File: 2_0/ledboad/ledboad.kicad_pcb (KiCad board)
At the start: 2 copper layers, 96 x 34.2 mm, 334 parts, among them J1 Conn_02x05_Odd_Even, Q1 AO3401A, Q2 AO3401A, Q3 AO3401A, Q4 AO3401A, Q5 AO3401A, Q6 AO3401A, Q7 AO3401A, Q8 AO3401A, SW1 RST, U1 STM32G070CBTx, U2 XC6206PxxxMR, Y1 2016/DNP

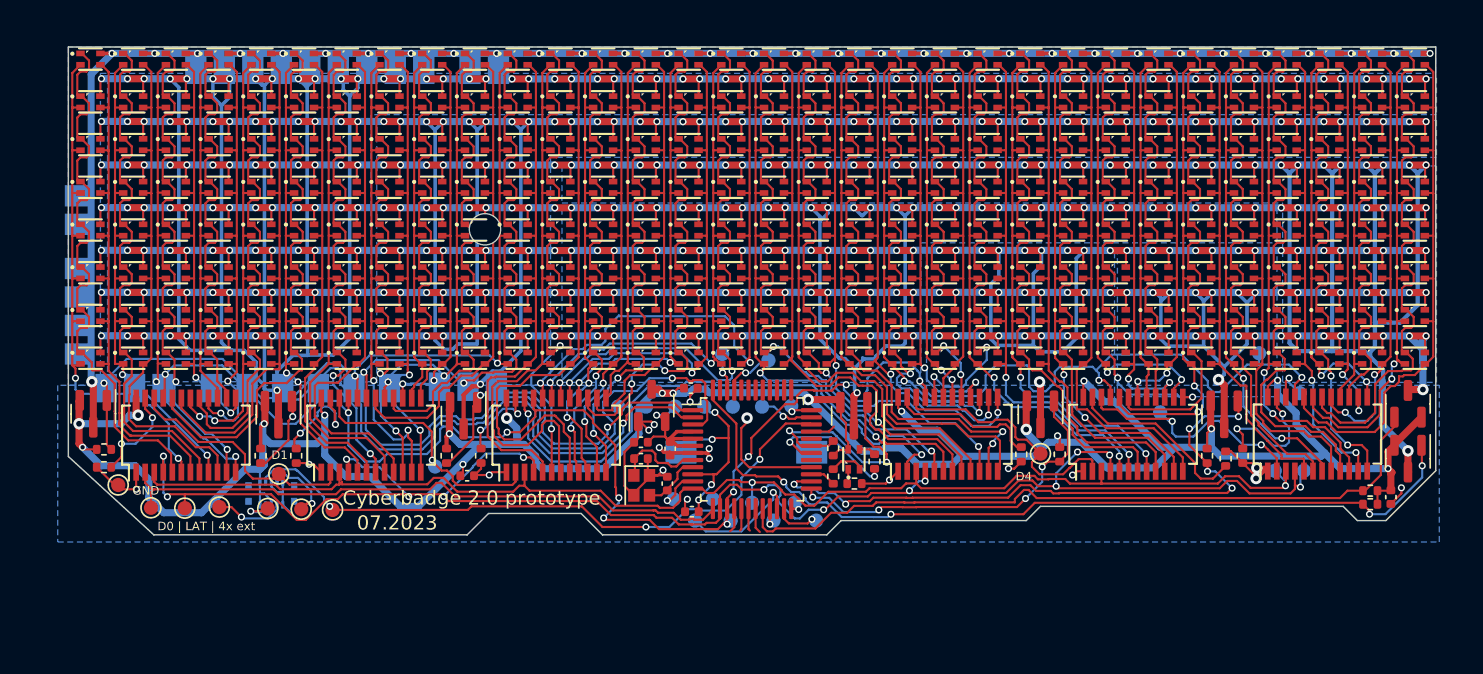
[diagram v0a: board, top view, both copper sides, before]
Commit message: commit before rescheme
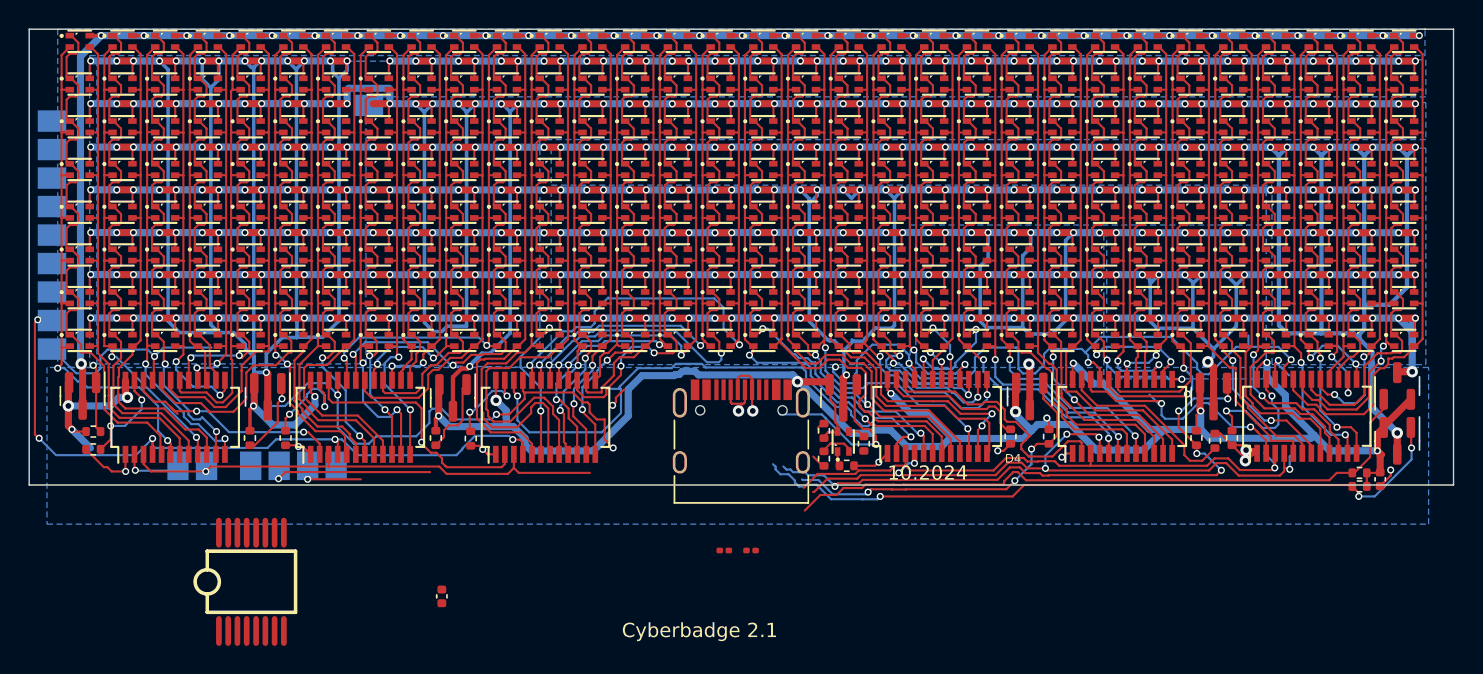
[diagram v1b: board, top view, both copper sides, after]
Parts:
- removed C1, C3: 100n, Capacitor_SMD:C_0402_1005Metric
- removed C2, C4: 470n, Capacitor_SMD:C_0402_1005Metric
- removed C7, C8: 10p/DNP, Capacitor_SMD:C_0402_1005Metric
- removed REF**: pilkbrain, Critbit_lib:pilkbrain
- removed SW1: RST, Button_Switch_SMD:SW_SPST_FSMSM
- removed TP1, TP10, TP11, TP12, TP13, TP14, TP15, TP16, TP17, TP18, TP19, TP2, TP20, TP21, TP22, TP23, TP24, TP25, TP26, TP27, TP28, TP29, TP3, TP30, TP31, TP32, TP4, TP5, TP6, TP7, TP8, TP9: TP, TestPoint:TestPoint_Pad_D1.0mm
- removed U1: STM32G070CBTx, Package_QFP:LQFP-48_7x7mm_P0.5mm
- removed Y1: 2016/DNP, Crystal:Crystal_SMD_2016-4Pin_2.0x1.6mm
- added R18: 5.1k, Resistor_SMD:R_0201_0603Metric, F.Cu at (93.7, 53.6)
- added R19: 5.1k, Resistor_SMD:R_0201_0603Metric, F.Cu at (91.8, 53.6)
- added U3: ~, Critbit_lib:pilkbrain, B.Cu at (55.8, 32.2)
- J1: value Conn_02x05_Odd_Even -> USB_C_Receptacle_USB2.0; footprint Critbit_lib:YXT-BB10-10S -> Connector_USB:USB_C_Receptacle_HRO_TYPE-C-31-M-12; moved to F.Cu
- U2: value XC6206PxxxMR -> 74HC138PW,118; footprint Package_TO_SOT_SMD:SOT-23-3 -> easyeda2kicad:SSOP-16_L6.2-W5.3-P0.65-LS7.8-BL
- moved J1 33.2 mm to (93.0, 46.4)
- moved U2 30.7 mm to (58.6, 55.8), turned to 0 degrees
- moved C5 8.66 mm to (72.0, 56.8), turned to 90 degrees
- moved C10 1.46 mm to (137.8, 48.6)
- moved D0_1 1.46 mm to (46.5, 17.9)
- moved D0_2 1.46 mm to (46.5, 20.8)
- moved D0_3 1.46 mm to (46.5, 23.8)
- moved D0_4 1.46 mm to (46.5, 26.8)
- moved D0_5 1.46 mm to (46.5, 29.8)
- moved D0_6 1.46 mm to (46.5, 32.8)
- moved D0_7 1.46 mm to (46.5, 35.8)
- moved D0_8 1.46 mm to (46.5, 38.8)
- moved D1 1.46 mm to (100.2, 46.0)
- moved D10_1 1.46 mm to (76.5, 17.9)
- moved D10_2 1.46 mm to (76.5, 20.8)
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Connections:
- RU6 pad 22: /DAT6 -> unconnected-(RU6-SDO-Pad22)
- U2 pad 1: GND -> /MATRIX_A
- U2 pad 2: +3V3 -> /MATRIX_B
- U2 pad 3: VDD -> /MATRIX_C
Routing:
- net /ROW_0_CTRL: track 67.2 -> 4.86 mm, vias 2 -> 1
- net /WS2812_DAT: track 45.1 -> 0.00 mm, vias 3 -> 0
- net VDD: track 195.9 -> 154.4 mm, vias 18 -> 15
- net /DAT0: track 44.2 -> 4.32 mm, vias 0 -> 1
- net /ROW_1_CTRL: track 46.5 -> 6.93 mm
- net GND: track 46.7 -> 21.0 mm, vias 17 -> 9
- net /OE: track 125.2 -> 100.4 mm, vias 12 -> 8
- net /LAT: track 119.6 -> 95.2 mm, vias 14 -> 11
- net /SCLK: track 93.6 -> 73.9 mm
- net /ROW_2_CTRL: track 24.9 -> 5.50 mm, vias 2 -> 0
- net /DM: track 0.00 -> 15.2 mm, vias 0 -> 2
- net /STM_NRST: track 14.2 -> 0.00 mm, vias 4 -> 0
- net +3V3: track 11.0 -> 0.00 mm, vias 1 -> 0
- net /ROW_3_CTRL: track 60.2 -> 50.3 mm, vias 4 -> 3
- net /STM_LEDB: track 9.66 -> 0.00 mm, vias 2 -> 0
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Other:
- board size 96 x 34.2 mm -> 100 x 32 mm
- board text added: "10.2024"
- board text added: "Cyberbadge 2.1"
- board text removed: "07.2023"
- board text removed: "Cyberbadge 2.0 prototype"
- board text removed: "D0 | LAT | 4x ext"
- board text removed: "D1"
- board text removed: "DAT2"
- board text removed: "DAT5"
- board text removed: "DAT6"
- board text removed: "GND"
- board text removed: "LAT | SCLK"
- board text removed: "OE"
- board text removed: "SPI2_MOSI | SPI2_MISO | OE | SPI2_SCLK"
- board text removed: "SPI2_NSS | SCLK | GND | ADC"
- board text removed: "SWCLK | SWDIO | GND | nRST | 3v3 | VDD | DAT3"
- board text removed: "TX | RX"
